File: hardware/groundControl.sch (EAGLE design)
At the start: 11 parts

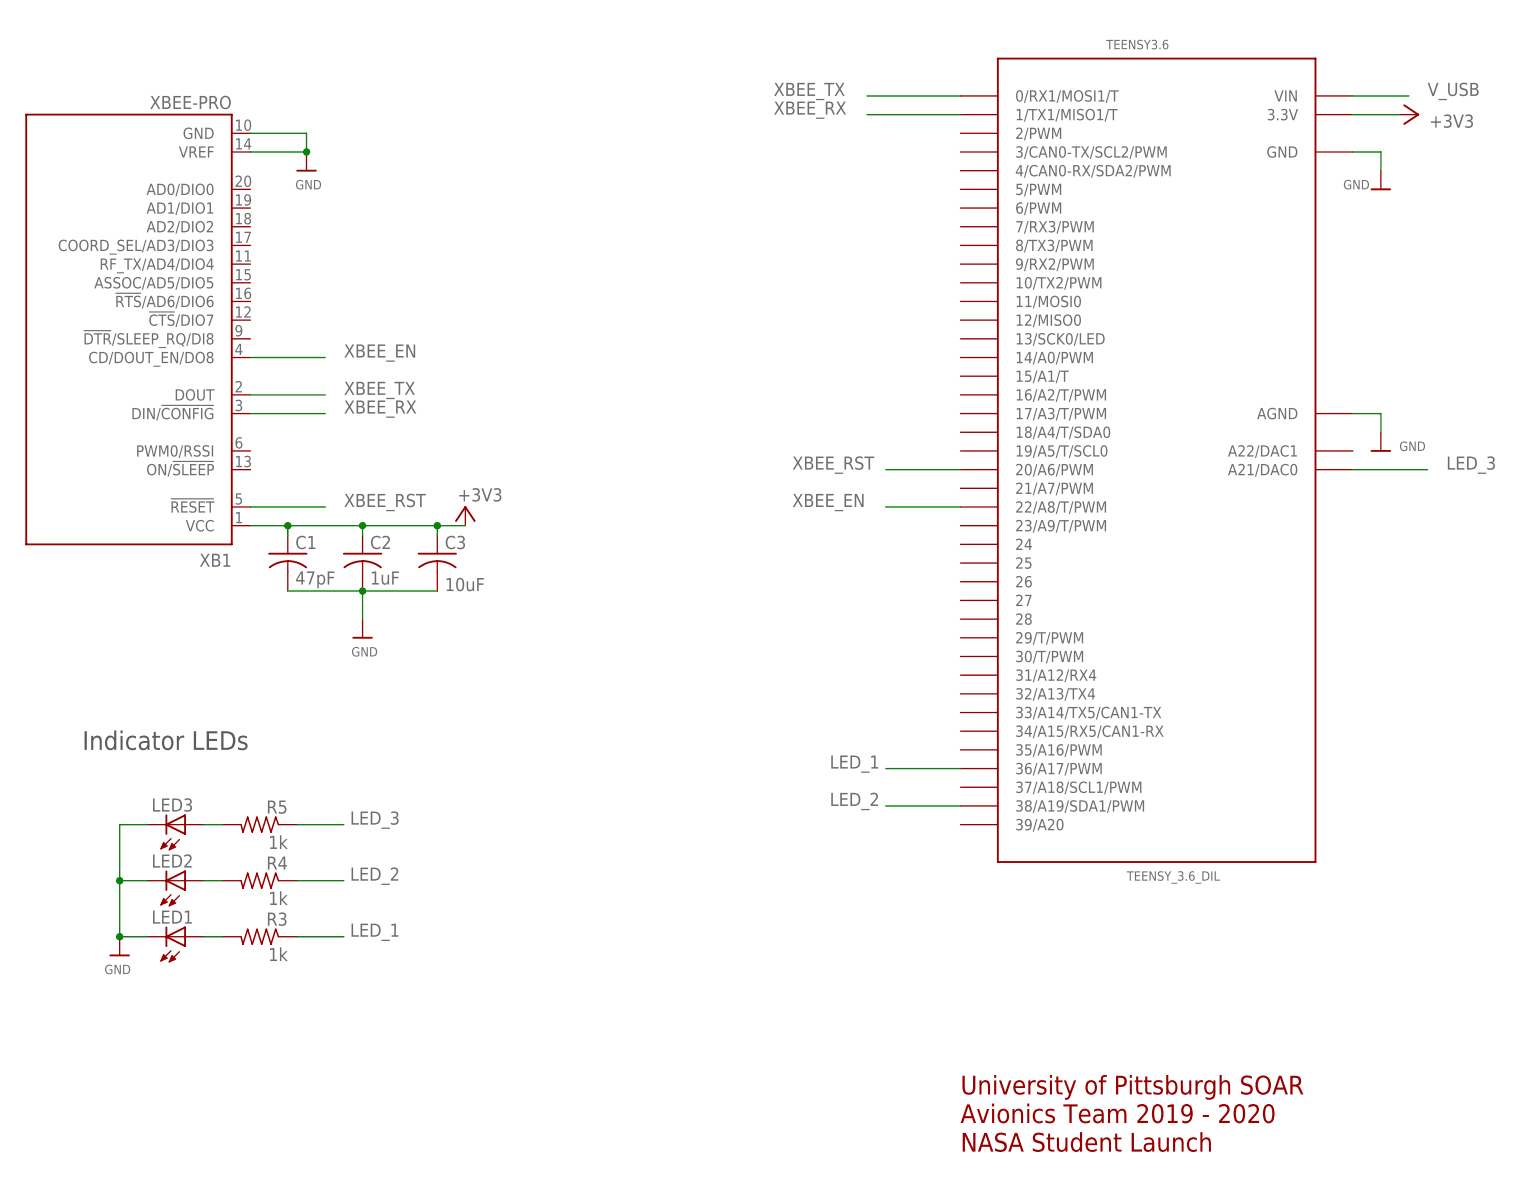
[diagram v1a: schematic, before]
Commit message: Teensy Change to 4.0
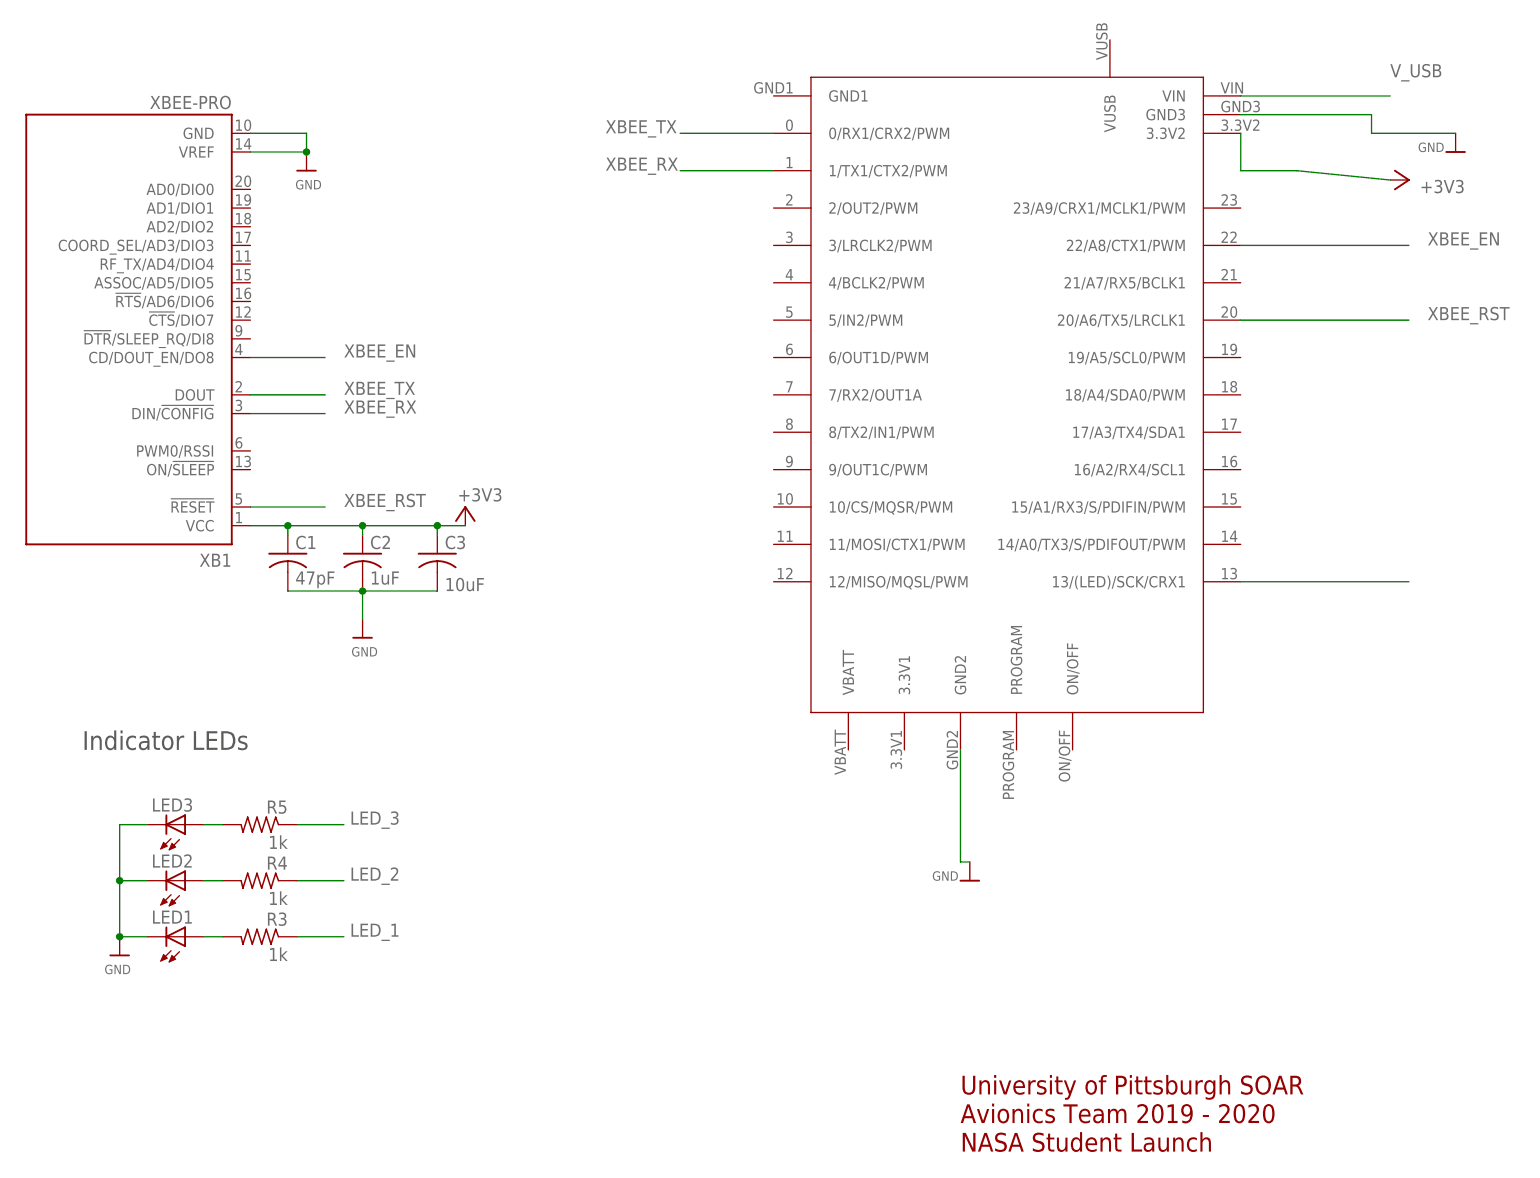
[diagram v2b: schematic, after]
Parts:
- removed TEENSY3.6: TEENSY_3.6_DIL, Teensy_3_and_LC_Series_Boards_v1.4:TEENSY_3.6_DIL
- added U$3: TEENSY4.0, Teensy 4.0:TEENSY4.0
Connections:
- new net N$11: U$3.13/(LED)/SCK/CRX1
- net +3V3: now also U$3.3.3V2; no longer TEENSY3.6.3.3V
- net GND: now also U$3.GND2, U$3.GND3; no longer TEENSY3.6.AGND, TEENSY3.6.GND
- net LED_1: no longer TEENSY3.6.36/A17/PWM
- net LED_2: no longer TEENSY3.6.38/A19/SDA1/PWM
- net LED_3: no longer TEENSY3.6.A21/DAC0
- net V_USB: now also U$3.VIN; no longer TEENSY3.6.VIN
- net XBEE_EN: now also U$3.22/A8/CTX1/PWM; no longer TEENSY3.6.22/A8/T/PWM
- net XBEE_RST: now also U$3.20/A6/TX5/LRCLK1; no longer TEENSY3.6.20/A6/PWM
- net XBEE_RX: now also U$3.1/TX1/CTX2/PWM; no longer TEENSY3.6.1/TX1/MISO1/T
- net XBEE_TX: now also U$3.0/RX1/CRX2/PWM; no longer TEENSY3.6.0/RX1/MOSI1/T
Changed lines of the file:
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@@
 <schematic_group name="XBEE"/>
 <schematic_group name="LED_BANK1"/>
+<schematic_group name="TEENSY_4.0"/>
 </groups>
 <parts>
-<part name="TEENSY3.6" library="Teensy_3_and_LC_Series_Boards_v1.4" deviceset="TEENSY_3.6_DIL" device=""/>
 <part name="FRAME2" library="frames" library_urn="urn:adsk.eagle:library:229" deviceset="A4L-LOC" device=""/>
 <part name="XB1" library="maxstream" library_urn="urn:adsk.eagle:library:270" deviceset="XBEE" device="-PRO" package3d_urn="urn:adsk.eagle:package:18008/1"/>
@@
 <part name="R5" library="resistor" library_urn="urn:adsk.eagle:library:348" deviceset="R-US_" device="0309/10" package3d_urn="urn:adsk.eagle:package:23567/1" value="1k"/>
 <part name="U$2" library="microbuilder" deviceset="GND" device=""/>
-<part name="+3V1" library="supply1" deviceset="+3V3" device=""/>
-<part name="U$14" library="microbuilder" deviceset="GND" device=""/>
-<part name="U$1" library="microbuilder" deviceset="GND" device=""/>
+<part name="U$3" library="Teensy 4.0" deviceset="TEENSY4.0" device=""/>
+<part name="+3V2" library="supply1" deviceset="+3V3" device=""/>
+<part name="U$4" library="microbuilder" deviceset="GND" device=""/>
+<part name="U$5" library="microbuilder" deviceset="GND" device=""/>
 </parts>
 <sheets>
@@
 </plain>
 <instances>
-<instance part="TEENSY3.6" gate="G$1" x="193.04" y="99.06" smashed="yes">
-<attribute name="NAME" x="184.912" y="156.21" size="1.27" layer="95" font="vector" ratio="15"/>
-<attribute name="VALUE" x="187.706" y="43.18" size="1.27" layer="96" font="vector" ratio="15"/>
-</instance>
 <instance part="FRAME2" gate="G$1" x="0" y="0" smashed="yes">
 <attribute name="DRAWING_NAME" x="217.17" y="15.24" size="2.54" layer="94"/>
@@
 <attribute name="VALUE" x="52.324" y="30.48" size="1.27" layer="96" rot="MR0"/>
 </instance>
-<instance part="+3V1" gate="G$1" x="227.33" y="147.32" smashed="yes" rot="R270">
-<attribute name="VALUE" x="234.95" y="147.32" size="1.778" layer="96" rot="R180"/>
-</instance>
-<instance part="U$14" gate="G$1" x="222.25" y="101.6" smashed="yes">
-<attribute name="VALUE" x="228.346" y="102.87" size="1.27" layer="96" rot="R180"/>
-</instance>
-<instance part="U$1" gate="G$1" x="222.25" y="137.16" smashed="yes">
-<attribute name="VALUE" x="220.726" y="138.43" size="1.27" layer="96" rot="R180"/>
+<instance part="U$3" gate="G$1" x="198.12" y="127" smashed="yes" grouprefs="TEENSY_4.0"/>
+<instance part="+3V2" gate="G$1" x="226.06" y="138.43" smashed="yes" rot="R270" grouprefs="TEENSY_4.0">
+<attribute name="VALUE" x="233.68" y="138.43" size="1.778" layer="96" rot="R180"/>
+</instance>
+<instance part="U$4" gate="G$1" x="232.41" y="142.24" smashed="yes" grouprefs="TEENSY_4.0">
+<attribute name="VALUE" x="230.886" y="143.51" size="1.27" layer="96" rot="R180"/>
+</instance>
+<instance part="U$5" gate="G$1" x="166.37" y="43.18" smashed="yes" grouprefs="TEENSY_4.0">
+<attribute name="VALUE" x="164.846" y="44.45" size="1.27" layer="96" rot="R180"/>
 </instance>
 </instances>
@@
 </segment>
 <segment>
-<pinref part="TEENSY3.6" gate="G$1" pin="AGND"/>
-<pinref part="U$14" gate="G$1" pin="GND"/>
-<wire x1="218.44" y1="106.68" x2="222.25" y2="106.68" width="0.1524" layer="91"/>
-<wire x1="222.25" y1="106.68" x2="222.25" y2="104.14" width="0.1524" layer="91"/>
-</segment>
-<segment>
-<pinref part="TEENSY3.6" gate="G$1" pin="GND"/>
-<pinref part="U$1" gate="G$1" pin="GND"/>
-<wire x1="218.44" y1="142.24" x2="222.25" y2="142.24" width="0.1524" layer="91"/>
-<wire x1="222.25" y1="142.24" x2="222.25" y2="139.7" width="0.1524" layer="91"/>
+<pinref part="U$3" gate="G$1" pin="GND3"/>
+<wire x1="203.2" y1="147.32" x2="220.98" y2="147.32" width="0.1524" layer="91" grouprefs="TEENSY_4.0"/>
+<pinref part="U$4" gate="G$1" pin="GND"/>
+<wire x1="220.98" y1="147.32" x2="220.98" y2="144.78" width="0.1524" layer="91" grouprefs="TEENSY_4.0"/>
+<wire x1="220.98" y1="144.78" x2="232.41" y2="144.78" width="0.1524" layer="91" grouprefs="TEENSY_4.0"/>
+</segment>
+<segment>
+<pinref part="U$3" gate="G$1" pin="GND2"/>
+<wire x1="165.1" y1="60.96" x2="165.1" y2="45.72" width="0.1524" layer="91" grouprefs="TEENSY_4.0"/>
+<pinref part="U$5" gate="G$1" pin="GND"/>
+<wire x1="166.37" y1="45.72" x2="165.1" y2="45.72" width="0.1524" layer="91" grouprefs="TEENSY_4.0"/>
 </segment>
 </net>
@@
 </segment>
 <segment>
-<pinref part="TEENSY3.6" gate="G$1" pin="3.3V"/>
-<pinref part="+3V1" gate="G$1" pin="+3V3"/>
-<wire x1="218.44" y1="147.32" x2="224.79" y2="147.32" width="0.1524" layer="91"/>
+<pinref part="U$3" gate="G$1" pin="3.3V2"/>
+<wire x1="203.2" y1="144.78" x2="203.2" y2="139.7" width="0.1524" layer="91" grouprefs="TEENSY_4.0"/>
+<wire x1="203.2" y1="139.7" x2="210.82" y2="139.7" width="0.1524" layer="91" grouprefs="TEENSY_4.0"/>
+<wire x1="210.82" y1="139.7" x2="223.52" y2="138.43" width="0.1524" layer="91" grouprefs="TEENSY_4.0"/>
+<pinref part="+3V2" gate="G$1" pin="+3V3"/>
 </segment>
 </net>
@@
 </segment>
 <segment>
-<pinref part="TEENSY3.6" gate="G$1" pin="1/TX1/MISO1/T"/>
-<wire x1="165.1" y1="147.32" x2="152.4" y2="147.32" width="0.1524" layer="91"/>
-<label x="139.7" y="147.32" size="1.778" layer="95"/>
+<pinref part="U$3" gate="G$1" pin="1/TX1/CTX2/PWM"/>
+<wire x1="139.7" y1="139.7" x2="127" y2="139.7" width="0.1524" layer="91" grouprefs="TEENSY_4.0"/>
+<label x="116.84" y="139.7" size="1.778" layer="95" grouprefs="TEENSY_4.0"/>
 </segment>
 </net>
@@
 </segment>
 <segment>
-<pinref part="TEENSY3.6" gate="G$1" pin="0/RX1/MOSI1/T"/>
-<wire x1="165.1" y1="149.86" x2="152.4" y2="149.86" width="0.1524" layer="91"/>
-<label x="139.7" y="149.86" size="1.778" layer="95"/>
+<pinref part="U$3" gate="G$1" pin="0/RX1/CRX2/PWM"/>
+<wire x1="139.7" y1="144.78" x2="127" y2="144.78" width="0.1524" layer="91" grouprefs="TEENSY_4.0"/>
+<label x="116.84" y="144.78" size="1.778" layer="95" grouprefs="TEENSY_4.0"/>
 </segment>
 </net>
@@
 </segment>
 <segment>
-<wire x1="165.1" y1="93.98" x2="154.94" y2="93.98" width="0.1524" layer="91"/>
-<pinref part="TEENSY3.6" gate="G$1" pin="22/A8/T/PWM"/>
-<label x="142.24" y="93.98" size="1.778" layer="95"/>
+<pinref part="U$3" gate="G$1" pin="22/A8/CTX1/PWM"/>
+<wire x1="203.2" y1="129.54" x2="226.06" y2="129.54" width="0.1524" layer="91" grouprefs="TEENSY_4.0"/>
+<label x="228.6" y="129.54" size="1.778" layer="95" grouprefs="TEENSY_4.0"/>
 </segment>
 </net>
@@
 </segment>
 <segment>
-<pinref part="TEENSY3.6" gate="G$1" pin="20/A6/PWM"/>
-<wire x1="165.1" y1="99.06" x2="154.94" y2="99.06" width="0.1524" layer="91"/>
-<label x="142.24" y="99.06" size="1.778" layer="95"/>
+<pinref part="U$3" gate="G$1" pin="20/A6/TX5/LRCLK1"/>
+<wire x1="203.2" y1="119.38" x2="226.06" y2="119.38" width="0.1524" layer="91" grouprefs="TEENSY_4.0"/>
+<label x="228.6" y="119.38" size="1.778" layer="95"/>
 </segment>
 </net>
@@
 <label x="88.9" y="50.8" size="1.778" layer="95" rot="MR0" grouprefs="LED_BANK1"/>
 </segment>
-<segment>
-<pinref part="TEENSY3.6" gate="G$1" pin="A21/DAC0"/>
-<wire x1="218.44" y1="99.06" x2="228.6" y2="99.06" width="0.1524" layer="91"/>
-<label x="231.14" y="99.06" size="1.778" layer="95"/>
-</segment>
 </net>
 <net name="LED_2" class="0">
@@
 <label x="88.9" y="43.18" size="1.778" layer="95" rot="MR0" grouprefs="LED_BANK1"/>
 </segment>
-<segment>
-<pinref part="TEENSY3.6" gate="G$1" pin="38/A19/SDA1/PWM"/>
-<wire x1="165.1" y1="53.34" x2="154.94" y2="53.34" width="0.1524" layer="91"/>
-<label x="147.32" y="53.34" size="1.778" layer="95"/>
-</segment>
 </net>
 <net name="LED_1" class="0">
@@
 <label x="88.9" y="35.56" size="1.778" layer="95" rot="MR0" grouprefs="LED_BANK1"/>
 </segment>
-<segment>
-<pinref part="TEENSY3.6" gate="G$1" pin="36/A17/PWM"/>
-<wire x1="165.1" y1="58.42" x2="154.94" y2="58.42" width="0.1524" layer="91"/>
-<label x="147.32" y="58.42" size="1.778" layer="95"/>
-</segment>
 </net>
 <net name="V_USB" class="0">
 <segment>
-<pinref part="TEENSY3.6" gate="G$1" pin="VIN"/>
-<wire x1="218.44" y1="149.86" x2="226.06" y2="149.86" width="0.1524" layer="91"/>
-<label x="228.6" y="149.86" size="1.778" layer="95"/>
-</segment>
-</net>
+<pinref part="U$3" gate="G$1" pin="VIN"/>
+<wire x1="203.2" y1="149.86" x2="223.52" y2="149.86" width="0.1524" layer="91" grouprefs="TEENSY_4.0"/>
+<label x="223.52" y="152.4" size="1.778" layer="95" grouprefs="TEENSY_4.0"/>
+</segment>
+</net>
+<net name="N$11" class="0">
+<segment>
+<pinref part="U$3" gate="G$1" pin="13/(LED)/SCK/CRX1"/>
+<wire x1="203.2" y1="83.82" x2="226.06" y2="83.82" width="0.1524" layer="91" grouprefs="TEENSY_4.0"/>
+</segment>
+</net>
